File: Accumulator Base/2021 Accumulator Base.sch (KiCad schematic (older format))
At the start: 58 parts, among them J1 Jumper, J10 Inverter&Motor, J11 Jumper, J12 EnergyMeter-OUT, J13 Dash, J14 Jumper, J15 Jumper, J16 Reset button, J17 Inverter-, J18 Jumper, J19 EnergyMeter-IN, J2 BMB, J3 TSMP, J4 Inv&Bat+, J5 Peripherals, J7 Interlocks, J8 Main LV, J9 AIRs, Q3 Q_NMOS_GDS, Q4 Q_NMOS_GDS, Q6 Q_NMOS_GDS, Q7 Q_NMOS_GDS, Q8 Q_NMOS_GDS, U1 74HC86, U2 IMD, U3 SDC-CUFR-Full-Library, U5 PWR_Transducer, U8 AIL&TSAL

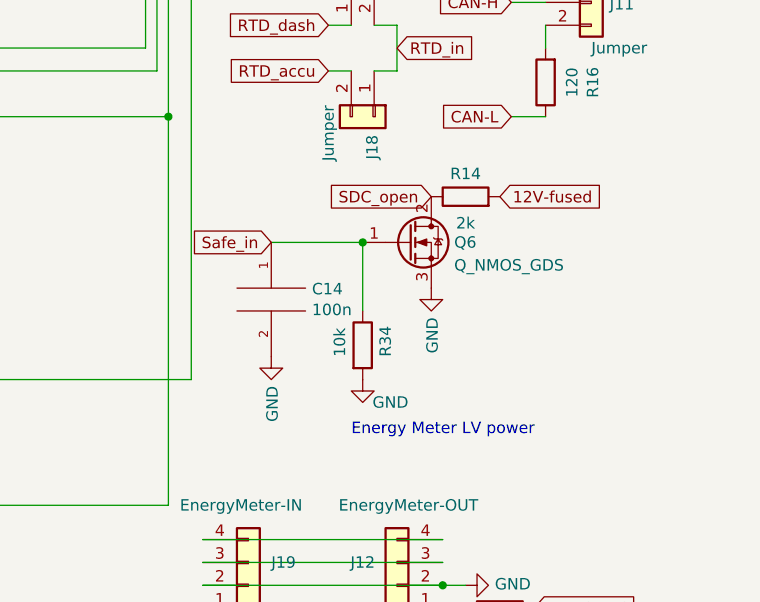
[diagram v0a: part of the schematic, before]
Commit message: Base PCB finished with traces
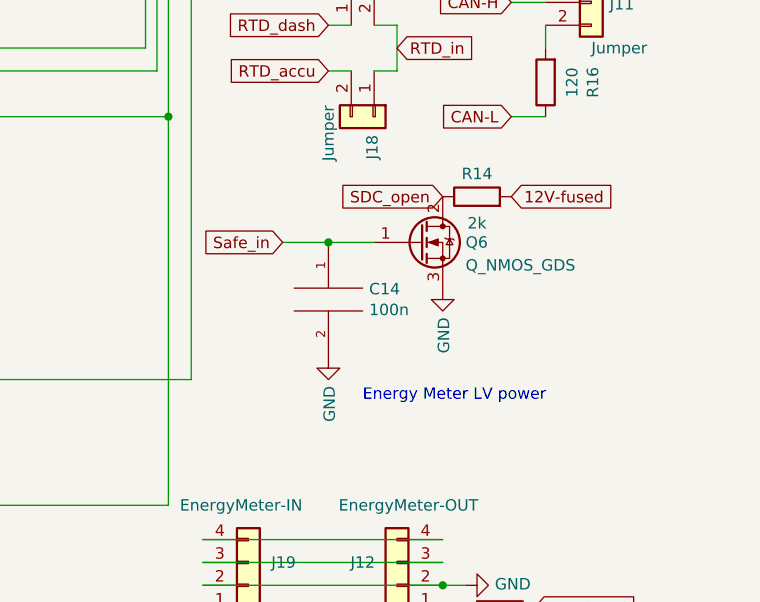
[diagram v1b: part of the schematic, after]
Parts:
- removed R34: 10k, Resistor_SMD:R_1206_3216Metric, symbol Device:R
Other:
- moved on the sheet: C14, Q6, R14
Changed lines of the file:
@@
 L Device:Q_NMOS_GDS Q?
 U 1 1 5F23AD1F
-P 10150 4750
+P 10200 4750
 AR Path="/5F13140A/5F23AD1F" Ref="Q?"  Part="1"
 AR Path="/5F23AD1F" Ref="Q6"  Part="1"
-F 0 "Q6" H 10350 4750 50  0000 L CNN
-F 1 "Q_NMOS_GDS" H 10350 4650 50  0000 L CNN
-F 2 "Package_TO_SOT_SMD:TO-252-2" H 10350 4850 50  0001 C CNN
-F 3 "~" H 10150 4750 50  0001 C CNN
-	1    10150 4750
+F 0 "Q6" H 10400 4750 50  0000 L CNN
+F 1 "Q_NMOS_GDS" H 10400 4650 50  0000 L CNN
+F 2 "Package_TO_SOT_SMD:TO-252-2" H 10400 4850 50  0001 C CNN
+F 3 "~" H 10200 4750 50  0001 C CNN
+	1    10200 4750
 	1    0    0    -1
 $EndComp
@@
 L power:GND #PWR?
 U 1 1 5F25E623
-P 10250 4950
+P 10300 4950
 AR Path="/5E8356A3/5F25E623" Ref="#PWR?"  Part="1"
 AR Path="/5F25E623" Ref="#PWR0102"  Part="1"
-F 0 "#PWR0102" H 10250 4700 50  0001 C CNN
-F 1 "GND" V 10255 4822 50  0000 R CNN
-F 2 "" H 10250 4950 50  0001 C CNN
-F 3 "" H 10250 4950 50  0001 C CNN
-	1    10250 4950
+F 0 "#PWR0102" H 10300 4700 50  0001 C CNN
+F 1 "GND" V 10305 4822 50  0000 R CNN
+F 2 "" H 10300 4950 50  0001 C CNN
+F 3 "" H 10300 4950 50  0001 C CNN
+	1    10300 4950
 	1    0    0    -1
 $EndComp
@@
 L Device:R R?
 U 1 1 5F28079E
-P 10400 4550
+P 10450 4550
 AR Path="/5E8356A3/5F28079E" Ref="R?"  Part="1"
 AR Path="/5F28079E" Ref="R14"  Part="1"
-F 0 "R14" V 10500 4550 50  0000 C CNN
-F 1 "2k" V 10284 4550 50  0000 C CNN
-F 2 "Resistor_SMD:R_1206_3216Metric" V 10330 4550 50  0001 C CNN
-F 3 "~" H 10400 4550 50  0001 C CNN
-	1    10400 4550
+F 0 "R14" V 10550 4550 50  0000 C CNN
+F 1 "2k" V 10334 4550 50  0000 C CNN
+F 2 "Resistor_SMD:R_1206_3216Metric" V 10380 4550 50  0001 C CNN
+F 3 "~" H 10450 4550 50  0001 C CNN
+	1    10450 4550
 	0    -1   -1   0
 $EndComp
-Text GLabel 10550 4550 2    50   Input ~ 0
+Text GLabel 10600 4550 2    50   Input ~ 0
 12V-fused
-Text GLabel 10250 4550 0    50   Input ~ 0
+Text GLabel 10300 4550 0    50   Input ~ 0
 SDC_open
 Text GLabel 4900 2750 0    50   Input ~ 0
@@
 Text GLabel 9450 1400 0    50   Input ~ 0
 SDC_open
-Text GLabel 9550 4750 0    50   Input ~ 0
+Text GLabel 9600 4750 0    50   Input ~ 0
 Safe_in
 $Comp
@@
 Text GLabel 10700 6350 2    50   Input ~ 0
 12V-fused
-Text Notes 9900 5600 0    50   ~ 0
+Text Notes 9950 5450 0    50   ~ 0
 Energy Meter LV power
 Text GLabel 7900 3200 2    50   Input ~ 0
@@
 L pspice:C C14
 U 1 1 5F4BB322
-P 9550 5000
-F 0 "C14" H 9728 5046 50  0000 L CNN
-F 1 "100n" H 9728 4955 50  0000 L CNN
-F 2 "Capacitor_SMD:C_0805_2012Metric" H 9550 5000 50  0001 C CNN
-F 3 "~" H 9550 5000 50  0001 C CNN
-	1    9550 5000
+P 9800 5000
+F 0 "C14" H 9978 5046 50  0000 L CNN
+F 1 "100n" H 9978 4955 50  0000 L CNN
+F 2 "Capacitor_SMD:C_0805_2012Metric" H 9800 5000 50  0001 C CNN
+F 3 "~" H 9800 5000 50  0001 C CNN
+	1    9800 5000
 	1    0    0    -1
 $EndComp
@@
 L power:GND #PWR?
 U 1 1 5F4BC1FA
-P 9550 5250
+P 9800 5250
 AR Path="/5E8356A3/5F4BC1FA" Ref="#PWR?"  Part="1"
 AR Path="/5F4BC1FA" Ref="#PWR0128"  Part="1"
-F 0 "#PWR0128" H 9550 5000 50  0001 C CNN
-F 1 "GND" V 9555 5122 50  0000 R CNN
-F 2 "" H 9550 5250 50  0001 C CNN
-F 3 "" H 9550 5250 50  0001 C CNN
-	1    9550 5250
+F 0 "#PWR0128" H 9800 5000 50  0001 C CNN
+F 1 "GND" V 9805 5122 50  0000 R CNN
+F 2 "" H 9800 5250 50  0001 C CNN
+F 3 "" H 9800 5250 50  0001 C CNN
+	1    9800 5250
 	1    0    0    -1
 $EndComp
@@
 	0    -1   -1   0
 $EndComp
-$Comp
-L Device:R R?
-U 1 1 5F4469E9
-P 9950 5200
-AR Path="/5F13151C/5F4469E9" Ref="R?"  Part="1"
-AR Path="/5F4469E9" Ref="R34"  Part="1"
-F 0 "R34" V 10050 5150 50  0000 L CNN
-F 1 "10k" V 9850 5150 50  0000 L CNN
-F 2 "Resistor_SMD:R_1206_3216Metric" V 9880 5200 50  0001 C CNN
-F 3 "~" H 9950 5200 50  0001 C CNN
-	1    9950 5200
-	1    0    0    -1
-$EndComp
-$Comp
-L power:GND #PWR?
-U 1 1 5F4483BC
-P 9950 5350
-AR Path="/5E8356A3/5F4483BC" Ref="#PWR?"  Part="1"
-AR Path="/5F4483BC" Ref="#PWR0137"  Part="1"
-F 0 "#PWR0137" H 9950 5100 50  0001 C CNN
-F 1 "GND" H 10150 5250 50  0000 R CNN
-F 2 "" H 9950 5350 50  0001 C CNN
-F 3 "" H 9950 5350 50  0001 C CNN
-	1    9950 5350
-	1    0    0    -1
-$EndComp
-Wire Wire Line
-	9550 4750 9950 4750
-Wire Wire Line
-	9950 5050 9950 4750
-Connection ~ 9950 4750
+Wire Wire Line
+	9600 4750 9800 4750
+Connection ~ 9800 4750
+Wire Wire Line
+	9800 4750 10000 4750
 $EndSCHEMATC
